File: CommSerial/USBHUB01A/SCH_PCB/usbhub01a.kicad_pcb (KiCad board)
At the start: 4 copper layers, 80.8 x 80.8 mm, 149 parts, among them CON1 BARREL_JACK, J1 JUMP_2x1, J10 JUMP_2x1, J11 JUMP_2x1, J12 JUMP_5X2, J13 USB3_A, J14 USB3_B, J15 USB3_A, J16 USB3_A, J17 USB3_A, J18 JUMP_3X2, J2 JUMP_2x1, J3 JUMP_2x1, J4 JUMP_2x1, J5 JUMP_2x1, J6 JUMP_2x1, J7 JUMP_2x1, J8 JUMP_2x1, J9 JUMP_2x1, M1 HOLE, M2 HOLE, M3 HOLE, M4 HOLE, SW1 SPST, U1 CAT24C04YI-GT3OSCT-ND, U2 TUSB8041IPAPRQ1, U3 TPS7A4533KTTR, U4 TPS74801RGWR, U5 TPS2001CDGN, U6 TPS2001CDGN, U7 TPS2001CDGN, U8 TPS2001CDGN, Y1 24MHz

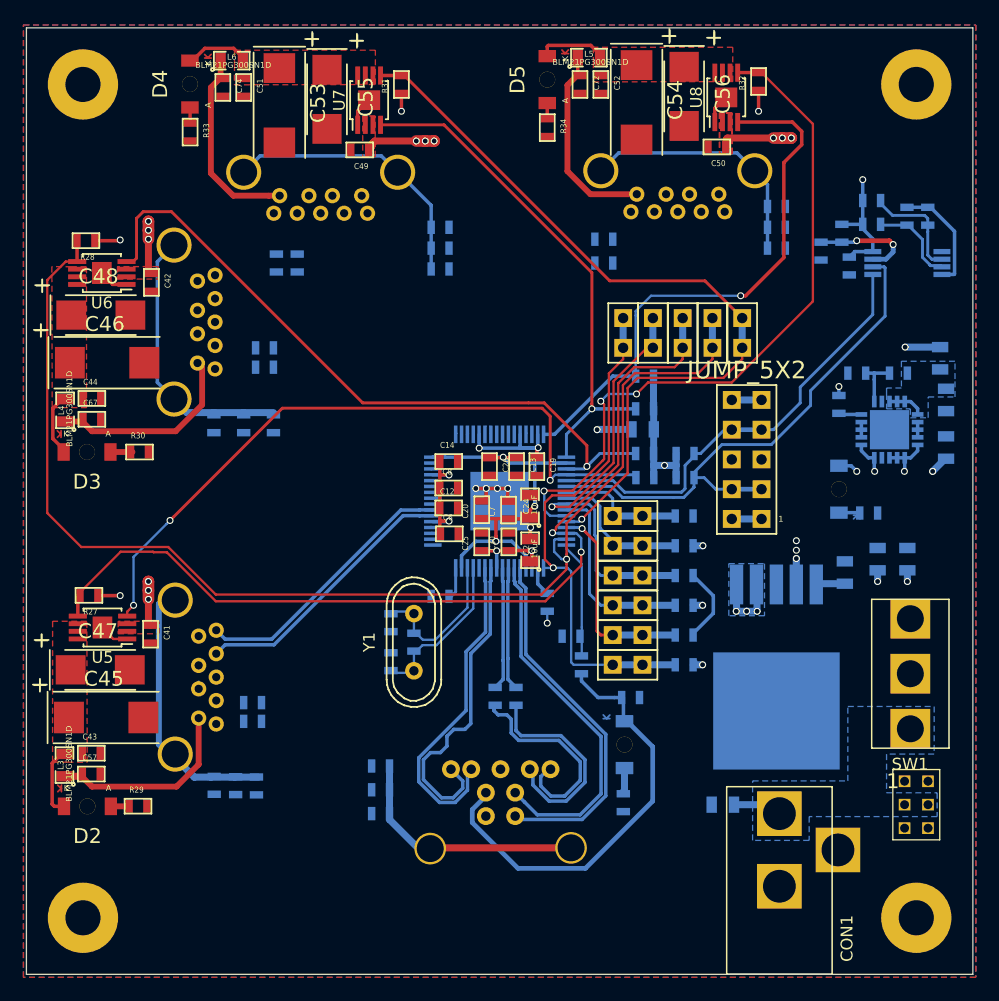
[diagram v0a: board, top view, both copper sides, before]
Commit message: První verze hotového layoutu
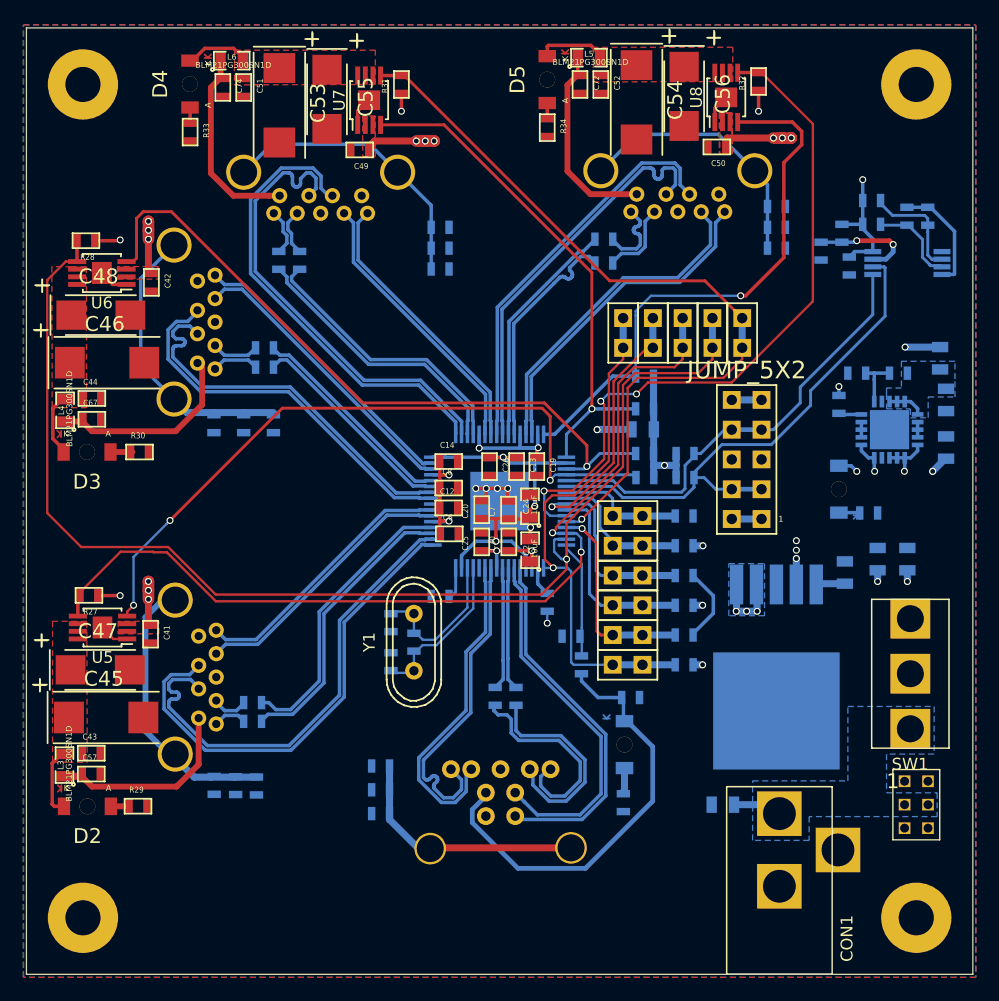
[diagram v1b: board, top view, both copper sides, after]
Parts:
- moved C79 0.31 mm to (130.3, 81.1)
- moved C80 0.31 mm to (128.5, 81.1)
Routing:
- net /USB_DM_DN1+: track 0.00 -> 41.3 mm
- net /USB_DM_DN1-: track 0.56 -> 41.4 mm
- net /USB_DM_DN3-: track 0.76 -> 40.6 mm
- net /USB_DM_DN3+: track 1.15 -> 41.0 mm
- net /USB_DM_DN4+: track 0.00 -> 34.3 mm
- net /USB_DM_DN4-: track 0.00 -> 34.3 mm
- net /USB_DM_DN2-: track 0.12 -> 33.4 mm
- net /USB_DM_DN2+: track 0.19 -> 33.5 mm
- net /USB_SSRXM_DN4+: track 0.17 -> 28.7 mm
- net /USB_SSRXM_DN4-: track 0.64 -> 28.8 mm
- net /USB_SSRXM_DN2+: track 0.19 -> 25.5 mm
- net /USB_SSRXM_DN2-: track 0.12 -> 25.4 mm
- net /USB_SSTXM_DN1+: track 0.61 -> 25.4 mm
- net /USB_SSTXM_DN1-: track 0.43 -> 25.2 mm
- net /USB_SSRXM_DN3+: track 1.32 -> 25.3 mm
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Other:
- net class Default: clearance 0.001 -> 0.1
- rule trace_clearance: 0.001 -> 0.1
